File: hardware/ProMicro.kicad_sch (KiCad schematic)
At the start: 22 parts, among them U3 ATMEGA32U4, Y1 16MHz

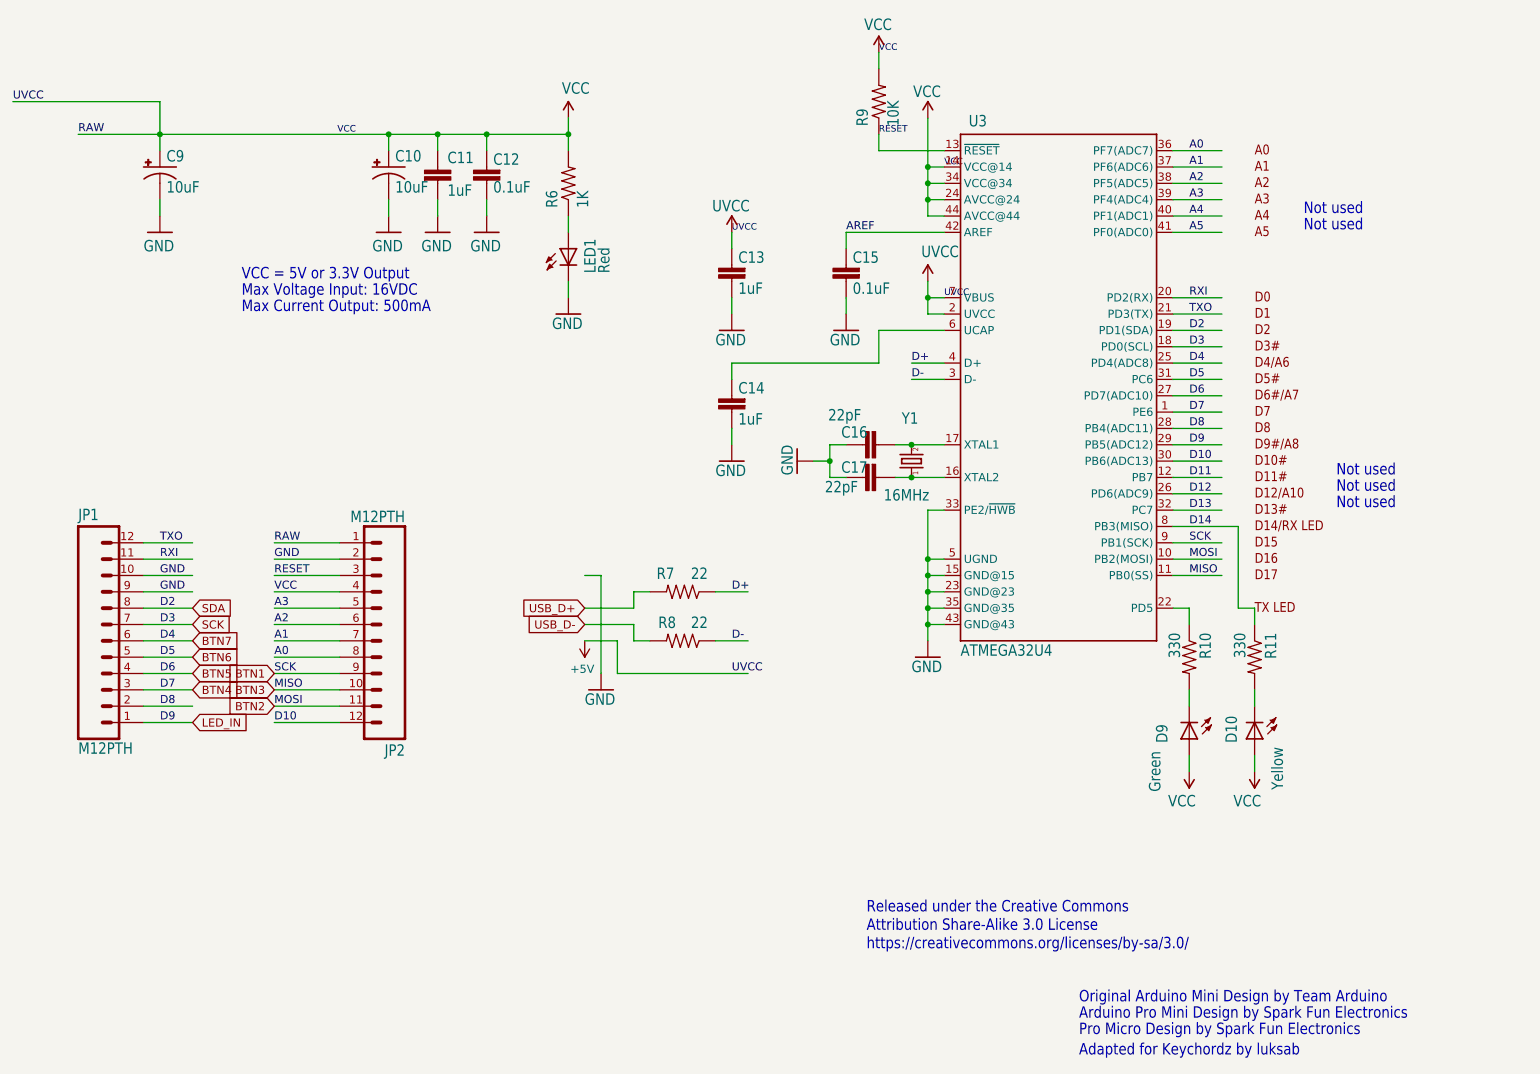
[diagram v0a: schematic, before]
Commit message: finish routing
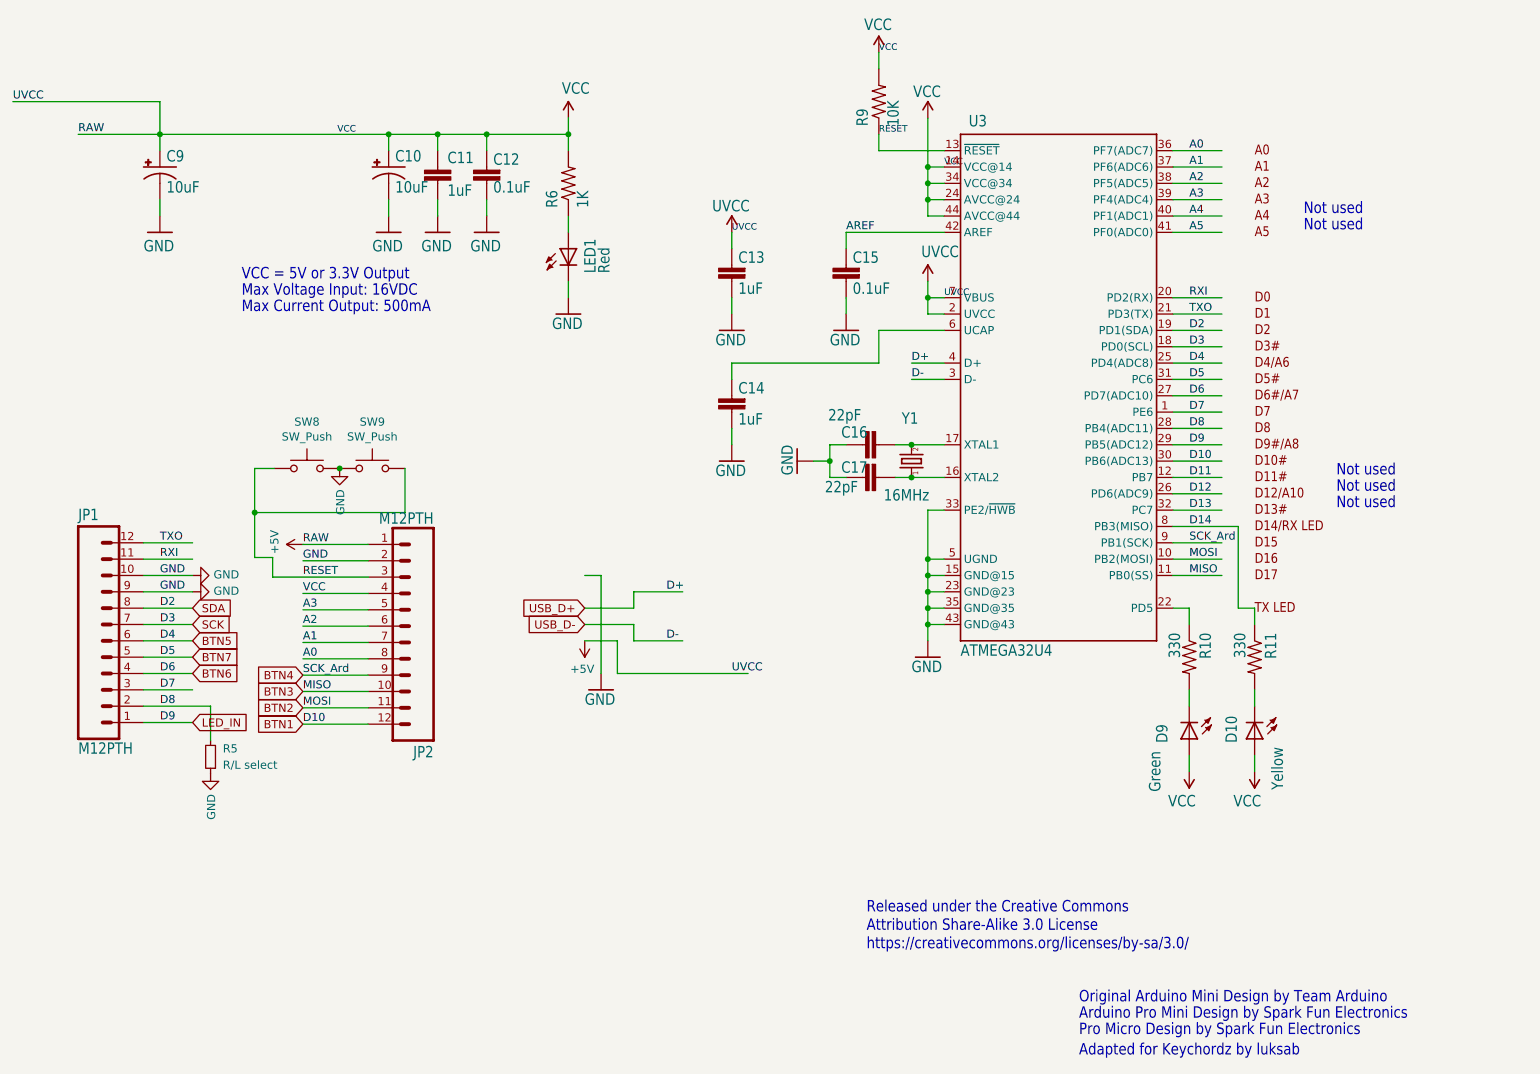
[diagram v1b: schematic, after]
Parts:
- removed R7, R8: 22, Resistor_SMD:R_0603_1608Metric_Pad0.98x0.95mm_HandSolder, symbol SparkFun_Pro_Micro-eagle-import:RESISTOR0603-RES
- added R5: R/L select, Resistor_SMD:R_0805_2012Metric_Pad1.20x1.40mm_HandSolder, symbol Device:R_Small
- added SW8, SW9: SW_Push, Button_Switch_SMD:SW_SPST_CK_RS282G05A3, symbol Switch:SW_Push
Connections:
- net D+ is gone; now on net USB_D+: U3.4 (D+)
- net D- is gone; now on net USB_D-: U3.3 (D-)
- net D10 is gone; now on net BTN1: JP2.12, U3.30 (PB6(ADC13))
- net BTN1: no longer JP1.7, JP2.9, U3.18 (PD0(SCL)), U3.9 (PB1(SCK))
- net BTN4: now also JP2.9, U3.9 (PB1(SCK)); no longer JP1.3, U3.1 (PE6)
- net BTN5: now also JP1.6, U3.25 (PD4(ADC8)); no longer JP1.4, U3.27 (PD7(ADC10))
- net BTN6: now also JP1.4, U3.27 (PD7(ADC10)); no longer JP1.5, U3.31 (PC6)
- net BTN7: now also JP1.5, U3.31 (PC6); no longer JP1.6, U3.25 (PD4(ADC8))
- net D8: now also R5.2
- net GND: now also R5.1, SW8.2, SW9.1
- net RESET: now also SW8.1, SW9.2
- new net D7: JP1.3, U3.1 (PE6)
- new net SCK: JP1.7, U3.18 (PD0(SCL))
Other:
- moved on the sheet: JP2
